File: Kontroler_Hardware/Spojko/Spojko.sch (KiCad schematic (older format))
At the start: 25 parts, among them J1 CONN_01X02, J2 CONN_01X06, P1 Raspberry_Pi, Q1 BSS138, Q2 BSS138, SW1 SW_Reset, SW2 SW_Flash, U1 ESP-12E, U6 DHT11

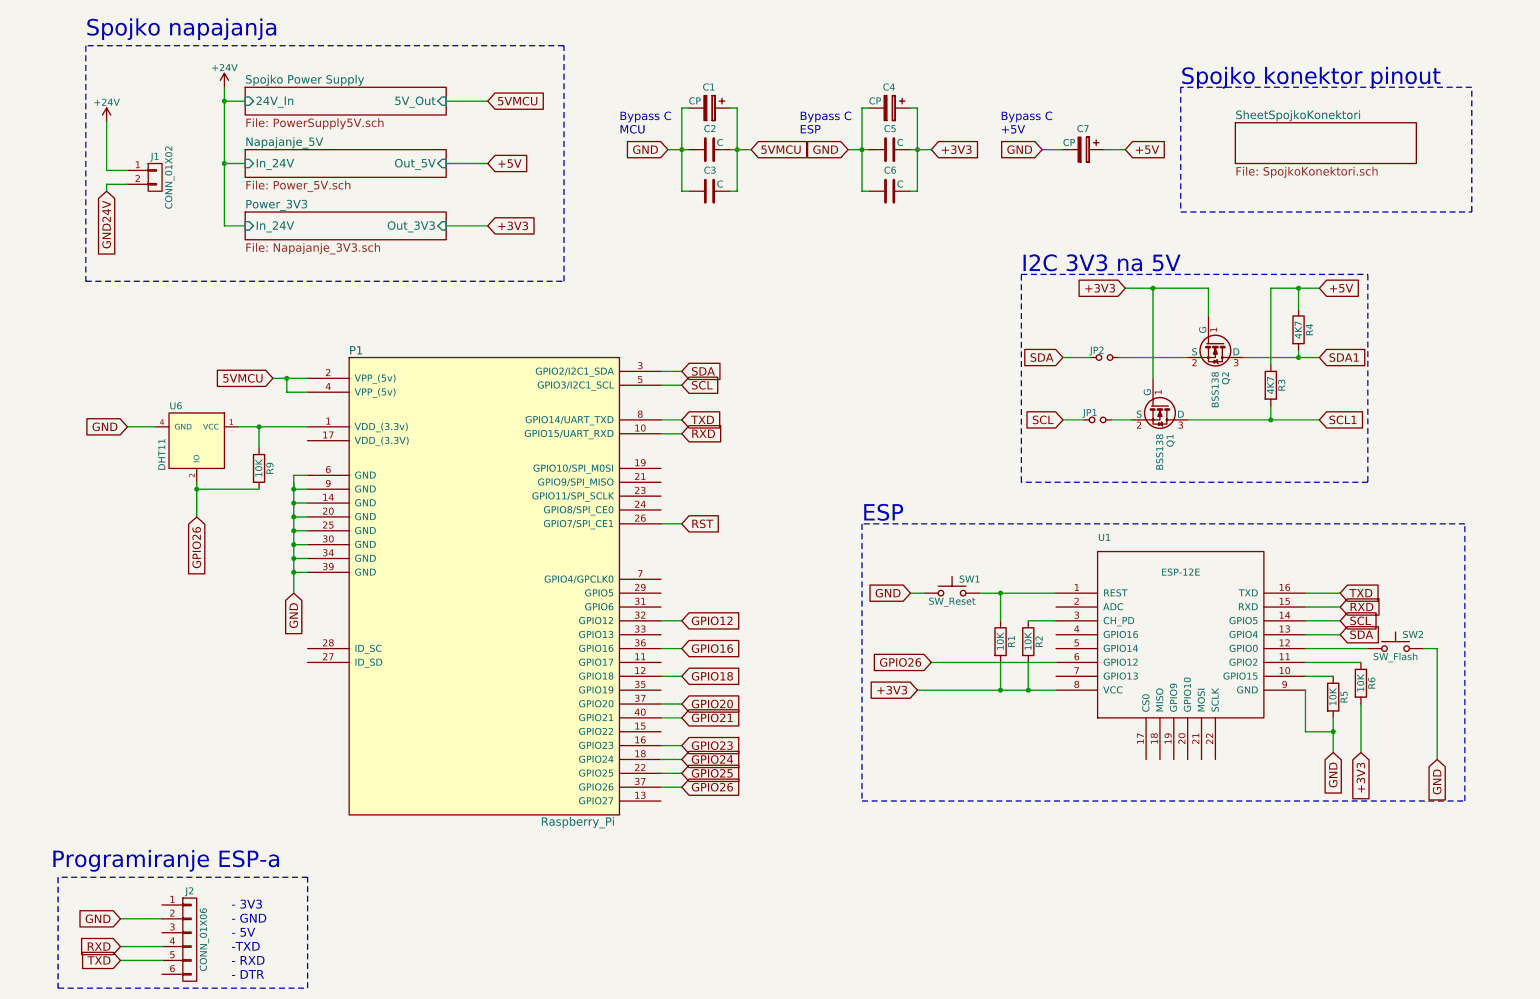
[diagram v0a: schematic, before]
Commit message: Nesto
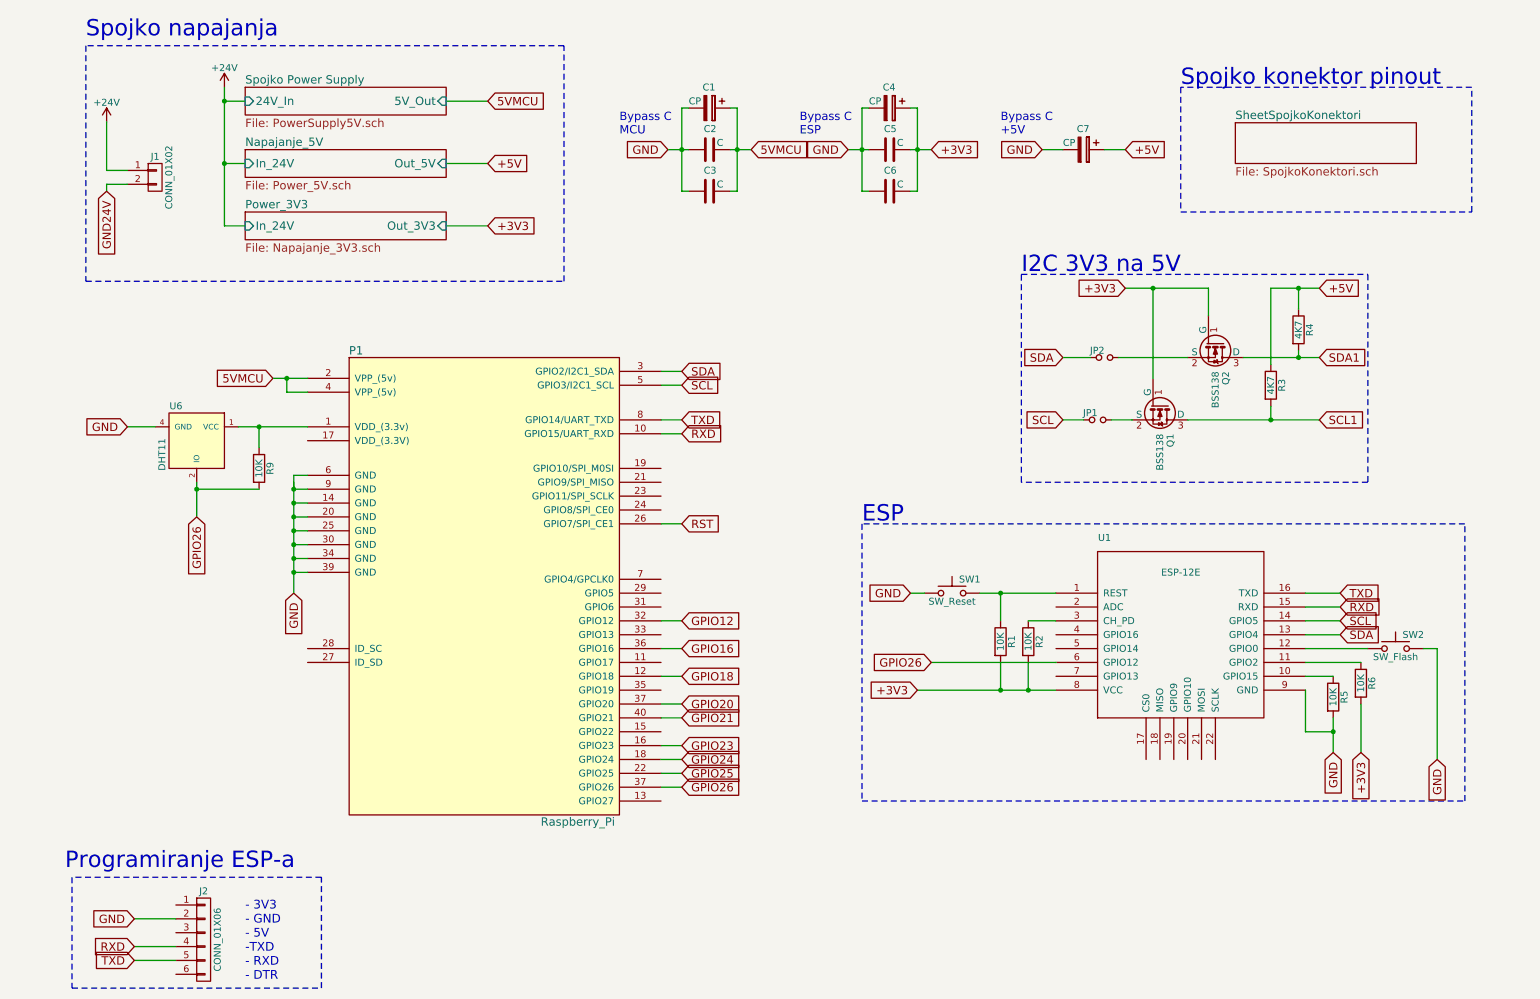
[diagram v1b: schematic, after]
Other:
- moved on the sheet: J2
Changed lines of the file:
@@
 L CONN_01X06 J2
 U 1 1 598FDB37
-P 1600 7200
-F 0 "J2" H 1600 7550 50  0000 C CNN
-F 1 "CONN_01X06" V 1700 7200 50  0000 C CNN
-F 2 "Pin_Headers:Pin_Header_Straight_1x06_Pitch2.54mm" H 1600 7200 50  0001 C CNN
-F 3 "" H 1600 7200 50  0001 C CNN
-	1    1600 7200
+P 1700 7200
+F 0 "J2" H 1700 7550 50  0000 C CNN
+F 1 "CONN_01X06" V 1800 7200 50  0000 C CNN
+F 2 "Pin_Headers:Pin_Header_Straight_1x06_Pitch2.54mm" H 1700 7200 50  0001 C CNN
+F 3 "" H 1700 7200 50  0001 C CNN
+	1    1700 7200
 	1    0    0    -1
 $EndComp
-Text Notes 1900 7500 0    63   ~ 0
+Text Notes 2000 7500 0    63   ~ 0
 - 3V3\n- GND\n- 5V\n-TXD\n- RXD\n- DTR
-Text GLabel 1100 7050 0    60   Input ~ 0
-GND
-Text GLabel 1100 7350 0    60   Input ~ 0
+Text GLabel 1200 7050 0    60   Input ~ 0
+GND
+Text GLabel 1200 7350 0    60   Input ~ 0
 TXD
-Text GLabel 1100 7250 0    60   Input ~ 0
+Text GLabel 1200 7250 0    60   Input ~ 0
 RXD
-Text Notes 600  6700 0    118  ~ 0
+Text Notes 700  6700 0    118  ~ 0
 Programiranje ESP-a\n
 Text Notes 6450 4200 0    118  ~ 0
@@
 	8300 3000 8800 3000
 Wire Wire Line
-	9200 3000 9750 3000
-Wire Wire Line
-	8800 3450 9750 3450
+	9200 3000 9600 3000
+Wire Wire Line
+	9600 3000 9750 3000
+Wire Wire Line
+	8800 3450 9400 3450
+Wire Wire Line
+	9400 3450 9750 3450
 Wire Wire Line
 	9400 3350 9400 3450
@@
 	9400 3050 9400 2500
 Wire Wire Line
-	9400 2500 9750 2500
+	9400 2500 9600 2500
+Wire Wire Line
+	9600 2500 9750 2500
 Wire Wire Line
 	9600 2650 9600 2500
 Connection ~ 9600 2500
 Wire Wire Line
-	8350 2500 8950 2500
+	8350 2500 8550 2500
+Wire Wire Line
+	8550 2500 8950 2500
 Wire Wire Line
 	8550 2500 8550 3150
@@
 	7450 4900 7450 4700
 Wire Wire Line
-	7300 4700 7850 4700
+	7300 4700 7450 4700
+Wire Wire Line
+	7450 4700 7850 4700
 Connection ~ 7450 4700
 Wire Wire Line
@@
 	9650 5700 9850 5700
 Wire Wire Line
-	9850 5600 9850 5850
+	9850 5600 9850 5700
+Wire Wire Line
+	9850 5700 9850 5850
 Connection ~ 9850 5700
 Wire Wire Line
 	9850 5300 9650 5300
 Wire Wire Line
-	1100 7050 1400 7050
-Wire Wire Line
-	1100 7250 1400 7250
-Wire Wire Line
-	1100 7350 1400 7350
-Wire Notes Line
-	650  6750 650  7550
-Wire Notes Line
-	650  7550 2450 7550
-Wire Notes Line
-	2450 7550 2450 6750
-Wire Notes Line
-	2450 6750 650  6750
+	1200 7050 1500 7050
+Wire Wire Line
+	1200 7250 1500 7250
+Wire Wire Line
+	1200 7350 1500 7350
+Wire Notes Line
+	750  6750 750  7550
+Wire Notes Line
+	750  7550 2550 7550
+Wire Notes Line
+	2550 7550 2550 6750
+Wire Notes Line
+	2550 6750 750  6750
 Wire Notes Line
 	10100 2400 10100 3900
@@
 	10850 1050 8750 1050
 Wire Wire Line
-	1950 3500 2450 3500
-Wire Wire Line
-	2350 3900 2350 4700
+	1950 3500 2100 3500
+Wire Wire Line
+	2100 3500 2450 3500
+Wire Wire Line
+	2350 3900 2350 3950
+Wire Wire Line
+	2350 3950 2350 4050
+Wire Wire Line
+	2350 4050 2350 4150
+Wire Wire Line
+	2350 4150 2350 4250
+Wire Wire Line
+	2350 4250 2350 4350
+Wire Wire Line
+	2350 4350 2350 4450
+Wire Wire Line
+	2350 4450 2350 4550
+Wire Wire Line
+	2350 4550 2350 4700
 Wire Wire Line
 	2350 3950 2350 3850
@@
 	2100 3950 1650 3950
 Wire Wire Line
-	1650 3900 1650 4150
+	1650 3900 1650 3950
+Wire Wire Line
+	1650 3950 1650 4150
 Connection ~ 1650 3950
 Wire Wire Line
@@
 	5200 1200 5150 1200
 Wire Wire Line
-	5150 1200 5150 1800
+	5150 1200 5150 1500
+Wire Wire Line
+	5150 1500 5150 1800
 Wire Wire Line
 	5150 1800 5200 1800
 Wire Wire Line
-	5050 1500 5200 1500
+	5050 1500 5150 1500
+Wire Wire Line
+	5150 1500 5200 1500
 Connection ~ 5150 1500
 Wire Wire Line
 	5500 1200 5550 1200
 Wire Wire Line
-	5550 1200 5550 1800
+	5550 1200 5550 1500
+Wire Wire Line
+	5550 1500 5550 1800
 Wire Wire Line
 	5550 1800 5500 1800
 Wire Wire Line
-	5500 1500 5650 1500
+	5500 1500 5550 1500
+Wire Wire Line
+	5550 1500 5650 1500
 Connection ~ 5550 1500
 Wire Wire Line
 	6500 1200 6450 1200
 Wire Wire Line
-	6450 1200 6450 1800
+	6450 1200 6450 1500
+Wire Wire Line
+	6450 1500 6450 1800
 Wire Wire Line
 	6450 1800 6500 1800
 Wire Wire Line
-	6350 1500 6500 1500
+	6350 1500 6450 1500
+Wire Wire Line
+	6450 1500 6500 1500
 Connection ~ 6450 1500
 Wire Wire Line
 	6800 1200 6850 1200
 Wire Wire Line
-	6850 1200 6850 1800
+	6850 1200 6850 1500
+Wire Wire Line
+	6850 1500 6850 1800
 Wire Wire Line
 	6850 1800 6800 1800
 Wire Wire Line
-	6800 1500 6950 1500
+	6800 1500 6850 1500
+Wire Wire Line
+	6850 1500 6950 1500
 Connection ~ 6850 1500
 Wire Wire Line
@@
 	8200 1500 8350 1500
 Wire Wire Line
-	2200 3150 2450 3150
+	2200 3150 2300 3150
+Wire Wire Line
+	2300 3150 2450 3150
 Wire Wire Line
 	2300 3250 2300 3150
@@
 	2000 1150 1850 1150
 Wire Wire Line
-	1850 1050 1850 2050
+	1850 1050 1850 1150
+Wire Wire Line
+	1850 1150 1850 1600
+Wire Wire Line
+	1850 1600 1850 2050
 Wire Wire Line
 	1850 2050 2000 2050
@@
 	6950 5200 7850 5200
 Wire Wire Line
-	6850 5400 7850 5400
+	6850 5400 7450 5400
+Wire Wire Line
+	7450 5400 7650 5400
+Wire Wire Line
+	7650 5400 7850 5400
 Wire Wire Line
 	10500 5100 10600 5100

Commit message: Change PowerConnector
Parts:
- J1: footprint Connectors:bornier2 -> Connectors_Phoenix:PhoenixContact_GMSTBA-G_02x7.62mm_Angled
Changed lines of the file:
@@
 F 0 "J1" H 1350 1850 50  0000 C CNN
 F 1 "CONN_01X02" V 1450 1700 50  0000 C CNN
-F 2 "Connectors:bornier2" H 1350 1700 50  0001 C CNN
+F 2 "Connectors_Phoenix:PhoenixContact_GMSTBA-G_02x7.62mm_Angled" H 1350 1700 50  0001 C CNN
 F 3 "" H 1350 1700 50  0001 C CNN
 	1    1350 1700
@@
 	8300 3000 8800 3000
 Wire Wire Line
-	9200 3000 9600 3000
-Wire Wire Line
-	9600 3000 9750 3000
-Wire Wire Line
-	8800 3450 9400 3450
-Wire Wire Line
-	9400 3450 9750 3450
+	9200 3000 9750 3000
+Wire Wire Line
+	8800 3450 9750 3450
 Wire Wire Line
 	9400 3350 9400 3450
@@
 	9400 3050 9400 2500
 Wire Wire Line
-	9400 2500 9600 2500
-Wire Wire Line
-	9600 2500 9750 2500
+	9400 2500 9750 2500
 Wire Wire Line
 	9600 2650 9600 2500
 Connection ~ 9600 2500
 Wire Wire Line
-	8350 2500 8550 2500
-Wire Wire Line
-	8550 2500 8950 2500
+	8350 2500 8950 2500
 Wire Wire Line
 	8550 2500 8550 3150
@@
 	7450 4900 7450 4700
 Wire Wire Line
-	7300 4700 7450 4700
-Wire Wire Line
-	7450 4700 7850 4700
+	7300 4700 7850 4700
 Connection ~ 7450 4700
 Wire Wire Line
@@
 	9650 5700 9850 5700
 Wire Wire Line
-	9850 5600 9850 5700
-Wire Wire Line
-	9850 5700 9850 5850
+	9850 5600 9850 5850
 Connection ~ 9850 5700
 Wire Wire Line
@@
 	10850 1050 8750 1050
 Wire Wire Line
-	1950 3500 2100 3500
-Wire Wire Line
-	2100 3500 2450 3500
-Wire Wire Line
-	2350 3900 2350 3950
-Wire Wire Line
-	2350 3950 2350 4050
-Wire Wire Line
-	2350 4050 2350 4150
-Wire Wire Line
-	2350 4150 2350 4250
-Wire Wire Line
-	2350 4250 2350 4350
-Wire Wire Line
-	2350 4350 2350 4450
-Wire Wire Line
-	2350 4450 2350 4550
-Wire Wire Line
-	2350 4550 2350 4700
+	1950 3500 2450 3500
+Wire Wire Line
+	2350 3900 2350 4700
 Wire Wire Line
 	2350 3950 2350 3850
@@
 	2100 3950 1650 3950
 Wire Wire Line
-	1650 3900 1650 3950
-Wire Wire Line
-	1650 3950 1650 4150
+	1650 3900 1650 4150
 Connection ~ 1650 3950
 Wire Wire Line
@@
 	5200 1200 5150 1200
 Wire Wire Line
-	5150 1200 5150 1500
-Wire Wire Line
-	5150 1500 5150 1800
+	5150 1200 5150 1800
 Wire Wire Line
 	5150 1800 5200 1800
 Wire Wire Line
-	5050 1500 5150 1500
-Wire Wire Line
-	5150 1500 5200 1500
+	5050 1500 5200 1500
 Connection ~ 5150 1500
 Wire Wire Line
 	5500 1200 5550 1200
 Wire Wire Line
-	5550 1200 5550 1500
-Wire Wire Line
-	5550 1500 5550 1800
+	5550 1200 5550 1800
 Wire Wire Line
 	5550 1800 5500 1800
 Wire Wire Line
-	5500 1500 5550 1500
-Wire Wire Line
-	5550 1500 5650 1500
+	5500 1500 5650 1500
 Connection ~ 5550 1500
 Wire Wire Line
 	6500 1200 6450 1200
 Wire Wire Line
-	6450 1200 6450 1500
-Wire Wire Line
-	6450 1500 6450 1800
+	6450 1200 6450 1800
 Wire Wire Line
 	6450 1800 6500 1800
 Wire Wire Line
-	6350 1500 6450 1500
-Wire Wire Line
-	6450 1500 6500 1500
+	6350 1500 6500 1500
 Connection ~ 6450 1500
 Wire Wire Line
 	6800 1200 6850 1200
 Wire Wire Line
-	6850 1200 6850 1500
-Wire Wire Line
-	6850 1500 6850 1800
+	6850 1200 6850 1800
 Wire Wire Line
 	6850 1800 6800 1800
 Wire Wire Line
-	6800 1500 6850 1500
-Wire Wire Line
-	6850 1500 6950 1500
+	6800 1500 6950 1500
 Connection ~ 6850 1500
 Wire Wire Line
@@
 	8200 1500 8350 1500
 Wire Wire Line
-	2200 3150 2300 3150
-Wire Wire Line
-	2300 3150 2450 3150
+	2200 3150 2450 3150
 Wire Wire Line
 	2300 3250 2300 3150
@@
 	2000 1150 1850 1150
 Wire Wire Line
-	1850 1050 1850 1150
-Wire Wire Line
-	1850 1150 1850 1600
-Wire Wire Line
-	1850 1600 1850 2050
+	1850 1050 1850 2050
 Wire Wire Line
 	1850 2050 2000 2050
@@
 	6950 5200 7850 5200
 Wire Wire Line
-	6850 5400 7450 5400
-Wire Wire Line
-	7450 5400 7650 5400
-Wire Wire Line
-	7650 5400 7850 5400
+	6850 5400 7850 5400
 Wire Wire Line
 	10500 5100 10600 5100
